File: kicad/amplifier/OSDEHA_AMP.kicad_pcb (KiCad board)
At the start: 2 copper layers, 89 parts, among them J1 INPUT, J2 HEATERS DC, J3 PSU HV, J4 OUTPUT, J5 DHT FIL2, J6 DHT FIL1, Q1 DN2540N5-G, Q10 DN2540, Q2 DN2540N5-G, Q3 STF3LN80K5, Q4 STF3LN80K5, Q5 AOT1N60, Q6 IXTP3N100D2, Q7 AOT1N60, Q8 IXTP3N100D2, Q9 DN2540, SW1 SW_DPDT_x2, U1 6E5P, U2 6E5P, U3 801A, U4 801A

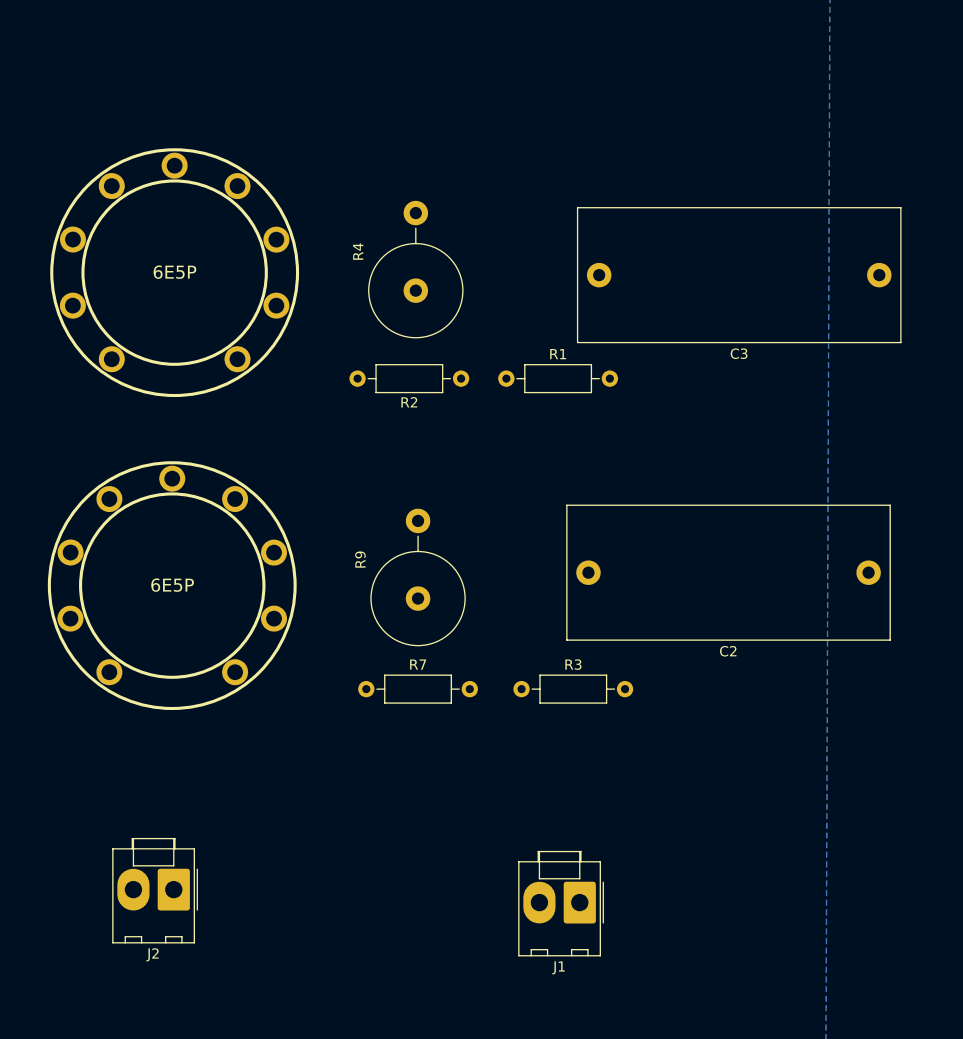
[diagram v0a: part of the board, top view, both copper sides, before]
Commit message: up
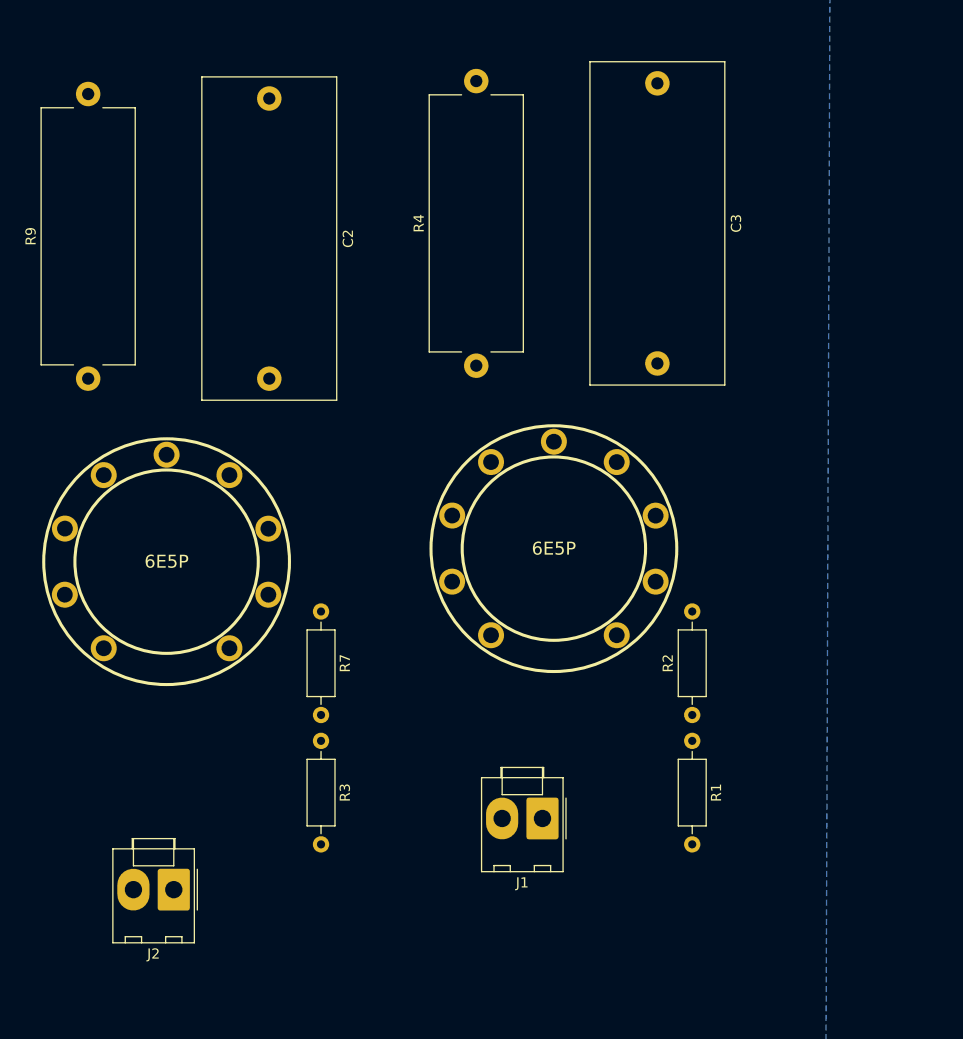
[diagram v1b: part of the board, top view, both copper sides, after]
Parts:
- R4, R9: footprint Resistor_THT:R_Axial_DIN0922_L20.0mm_D9.0mm_P7.62mm_Vertical -> Resistor_THT:R_Axial_Power_L25.0mm_W9.0mm_P27.94mm
- moved C2 75.0 mm to (-83.8, 61.4), turned to -90 degrees
- moved U1 46.0 mm to (-55.9, 105.6)
- moved R2 40.1 mm to (-42.3, 121.9), turned to 90 degrees
- moved R1 40.0 mm to (-42.3, 124.5), turned to -90 degrees
- moved R9 38.9 mm to (-101.6, 88.9)
- moved C3 28.8 mm to (-45.7, 59.9), turned to -90 degrees
- moved R3 20.3 mm to (-78.7, 124.5), turned to -90 degrees
- moved R4 9.46 mm to (-63.5, 87.6)
- moved J1 9.03 mm to (-57.0, 132.1)
- moved R7 8.82 mm to (-78.7, 111.8), turned to -90 degrees
- moved U2 2.41 mm to (-93.9, 106.9)
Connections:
- C6 pad 2: /Buffer_CCS_load1/NEG -> Net-(J3-Pin_3)
- C7 pad 2: Net-(J3-Pin_3) -> /Buffer_CCS_load1/NEG
